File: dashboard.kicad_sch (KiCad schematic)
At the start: 35 parts, among them J2 Conn_01x02, J3 RJ45, J4 Conn_01x10, J5 776267-1, Q1 2N7002, SW1 SW_Push, SW2 SW_SPST, SW4 SW_SPST, U1 TPS542025DDC, U2 R-78C5.0-1.0, U4 ILD74

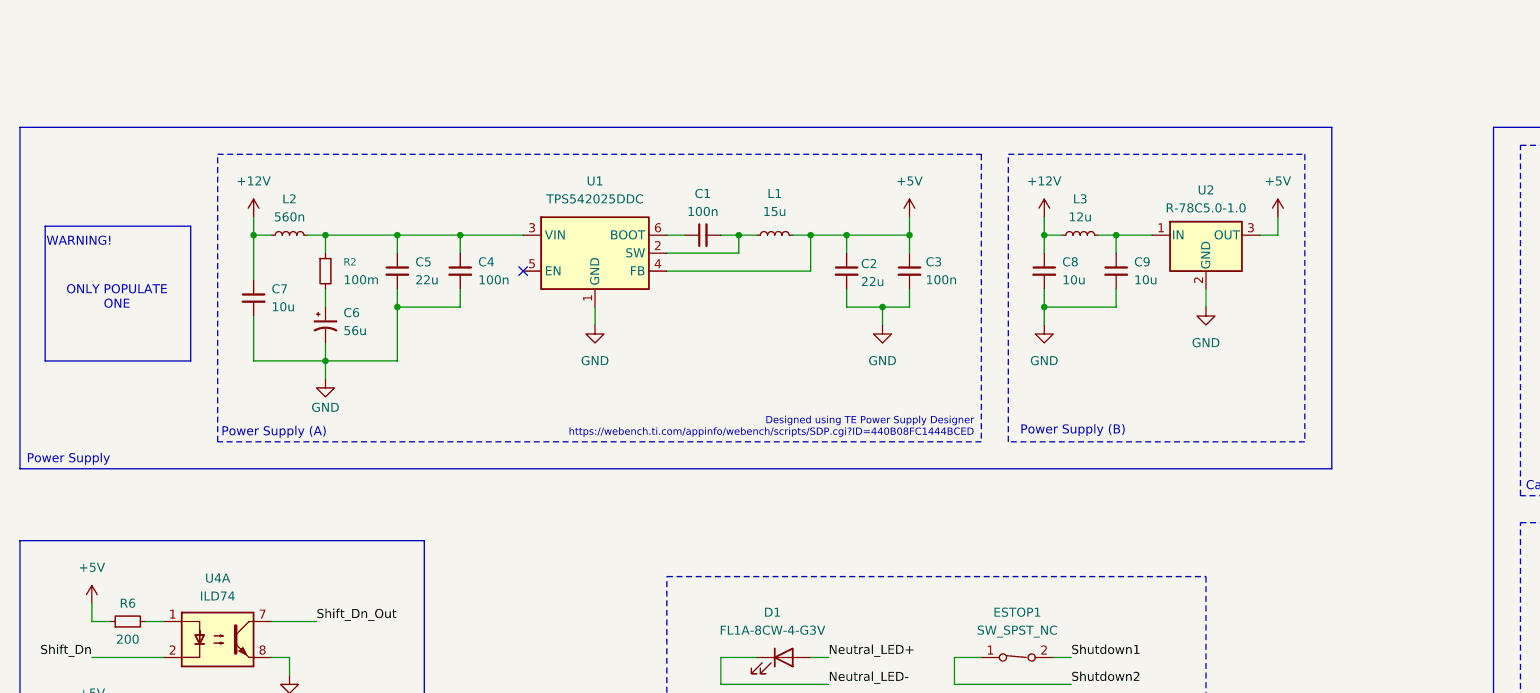
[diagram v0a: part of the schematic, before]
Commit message: Add power supply protection
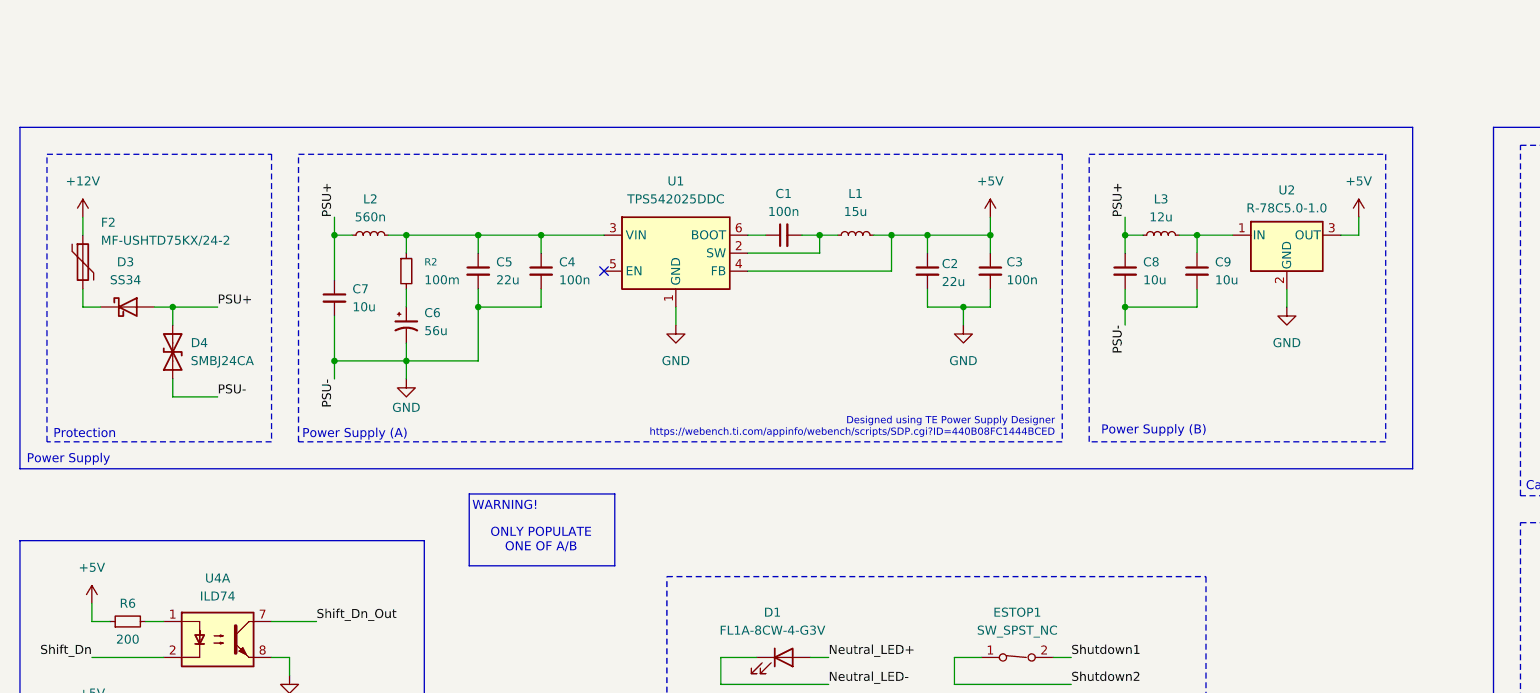
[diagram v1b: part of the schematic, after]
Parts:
- added D3: SS34, Diode_SMD:D_SMA, symbol Diode:SS34
- added D4: SMBJ24CA, Diode_SMD:D_SMB_Handsoldering, symbol Device:D_TVS
- added F2: MF-USHTD75KX/24-2, Fuse:Fuse_1210_3225Metric_Pad1.42x2.65mm_HandSolder, symbol Device:Polyfuse
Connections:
- net +12V: now also F2.1; no longer C7.1, C8.1, L2.1, L3.1
- net GND: now also D4.1 (A1)
- new net: D3.1 (K), F2.2
- new net PSU+: C7.1, C8.1, D3.2 (A), D4.2 (A2), L2.1, L3.1
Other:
- note added: "ONLY POPULATE ONE OF A/B"
- note added: "Protection"
- note removed: "ONLY POPULATE ONE"
- moved on the sheet: C1, C2, C3, C4, C5, C6, C7, C8, C9, L1, L2, L3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

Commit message: Revert "Add power supply protection"
This reverts commit 6c38df0548b9625adbd3b6c051cb9005b09ba150.
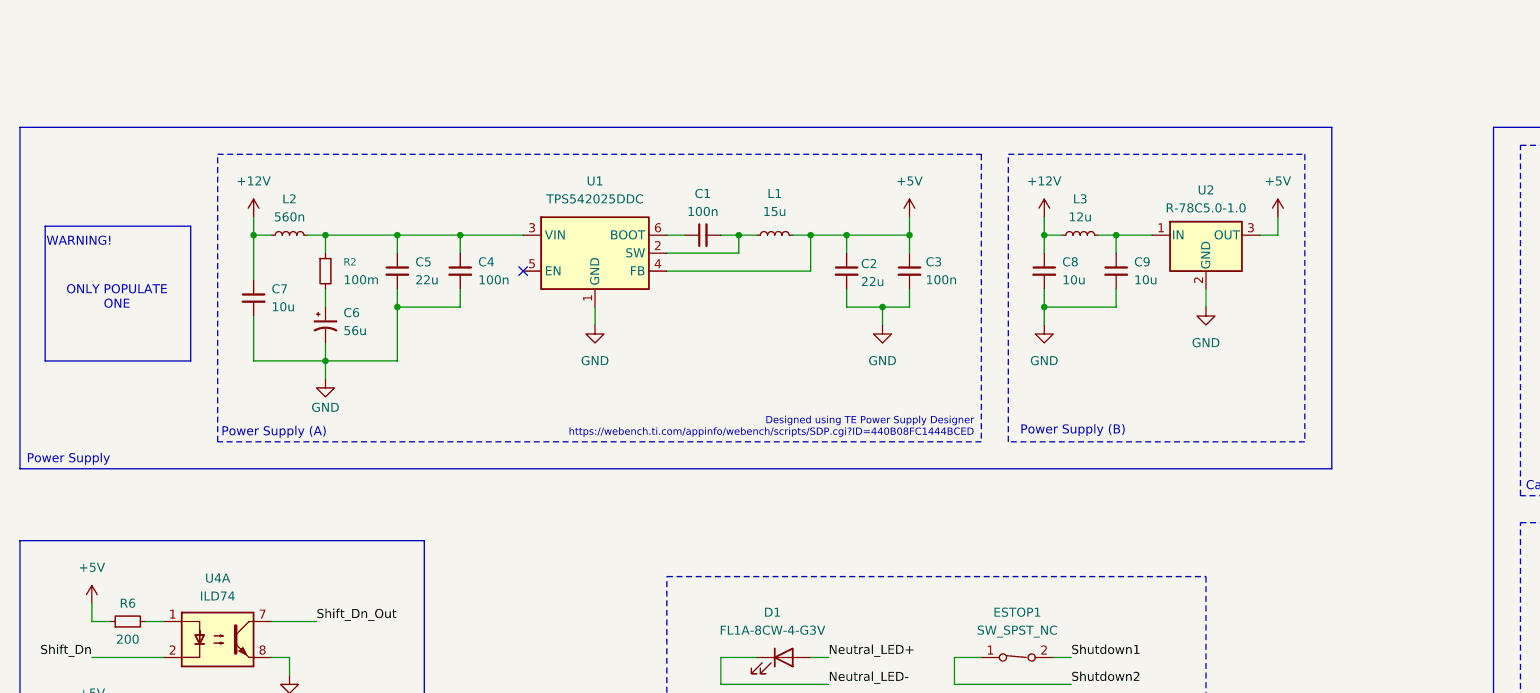
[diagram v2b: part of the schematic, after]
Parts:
- removed D3: SS34, Diode_SMD:D_SMA, symbol Diode:SS34
- removed D4: SMBJ24CA, Diode_SMD:D_SMB_Handsoldering, symbol Device:D_TVS
- removed F2: MF-USHTD75KX/24-2, Fuse:Fuse_1210_3225Metric_Pad1.42x2.65mm_HandSolder, symbol Device:Polyfuse
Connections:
- net PSU+ is gone; now on net +12V: C7.1, C8.1, L2.1, L3.1
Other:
- note added: "ONLY POPULATE ONE"
- note removed: "ONLY POPULATE ONE OF A/B"
- note removed: "Protection"
- moved on the sheet: C1, C2, C3, C4, C5, C6, C7, C8, C9, L1, L2, L3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
